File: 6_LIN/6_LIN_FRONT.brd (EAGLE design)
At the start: 71.5 x 24 mm, 3 parts

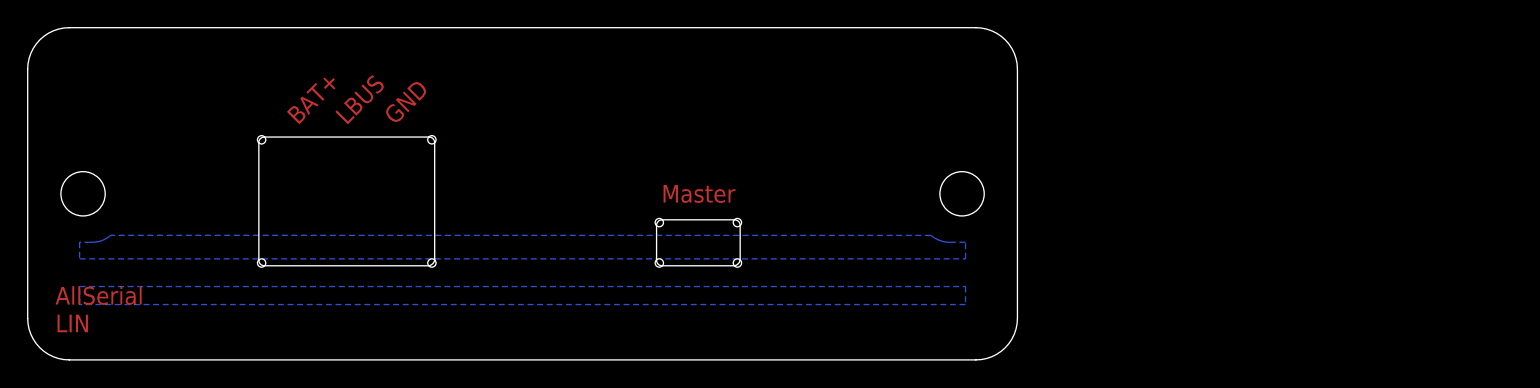
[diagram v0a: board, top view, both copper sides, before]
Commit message: Cleanup, front with lib elements
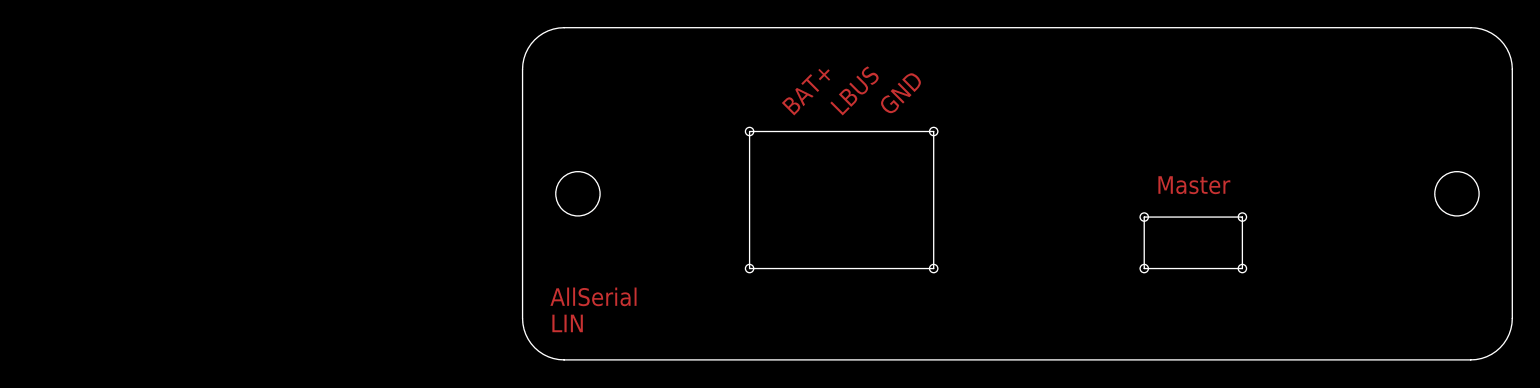
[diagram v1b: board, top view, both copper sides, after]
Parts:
- removed E$1: (no value), AllSerialv2:PANEL
- removed E$2: (no value), AllSerialv2:RIA_AKL182-03
- removed E$3: (no value), AllSerialv2:LSTB-02-1
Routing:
- removed copper zone on layer 16, net S$1
- removed copper zone on layer 16, net S$2
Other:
- outline, holes or cut-outs redrawn
- board text added: "AllSerial LIN"
- board text removed: "AllSerial - LIN v1.2 46/18"
- board text removed: "LIN"
